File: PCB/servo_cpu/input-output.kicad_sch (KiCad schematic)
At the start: 1 part, among them J8 IO

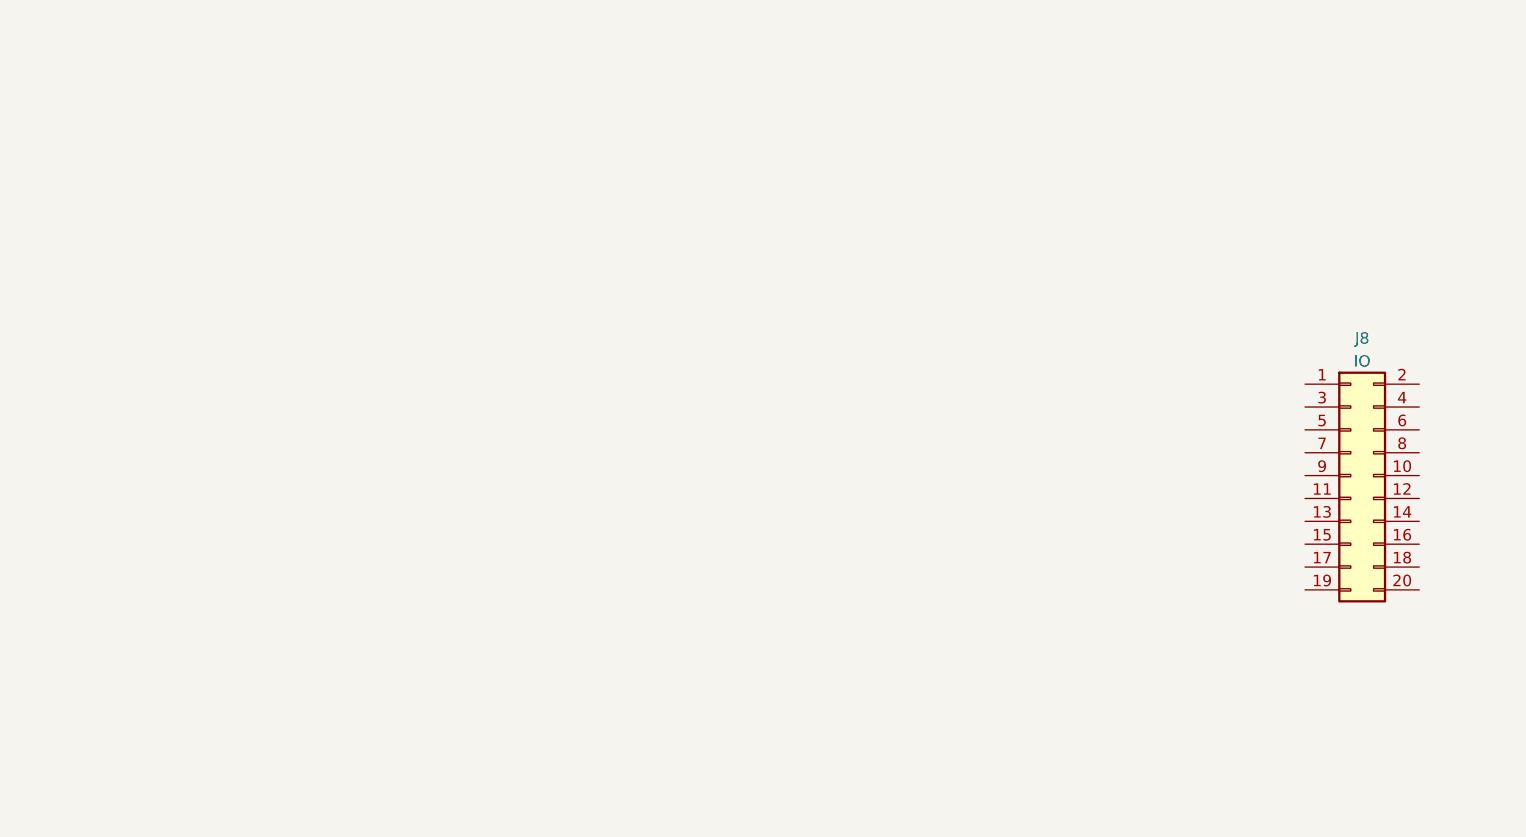
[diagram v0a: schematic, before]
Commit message: cpu pcb
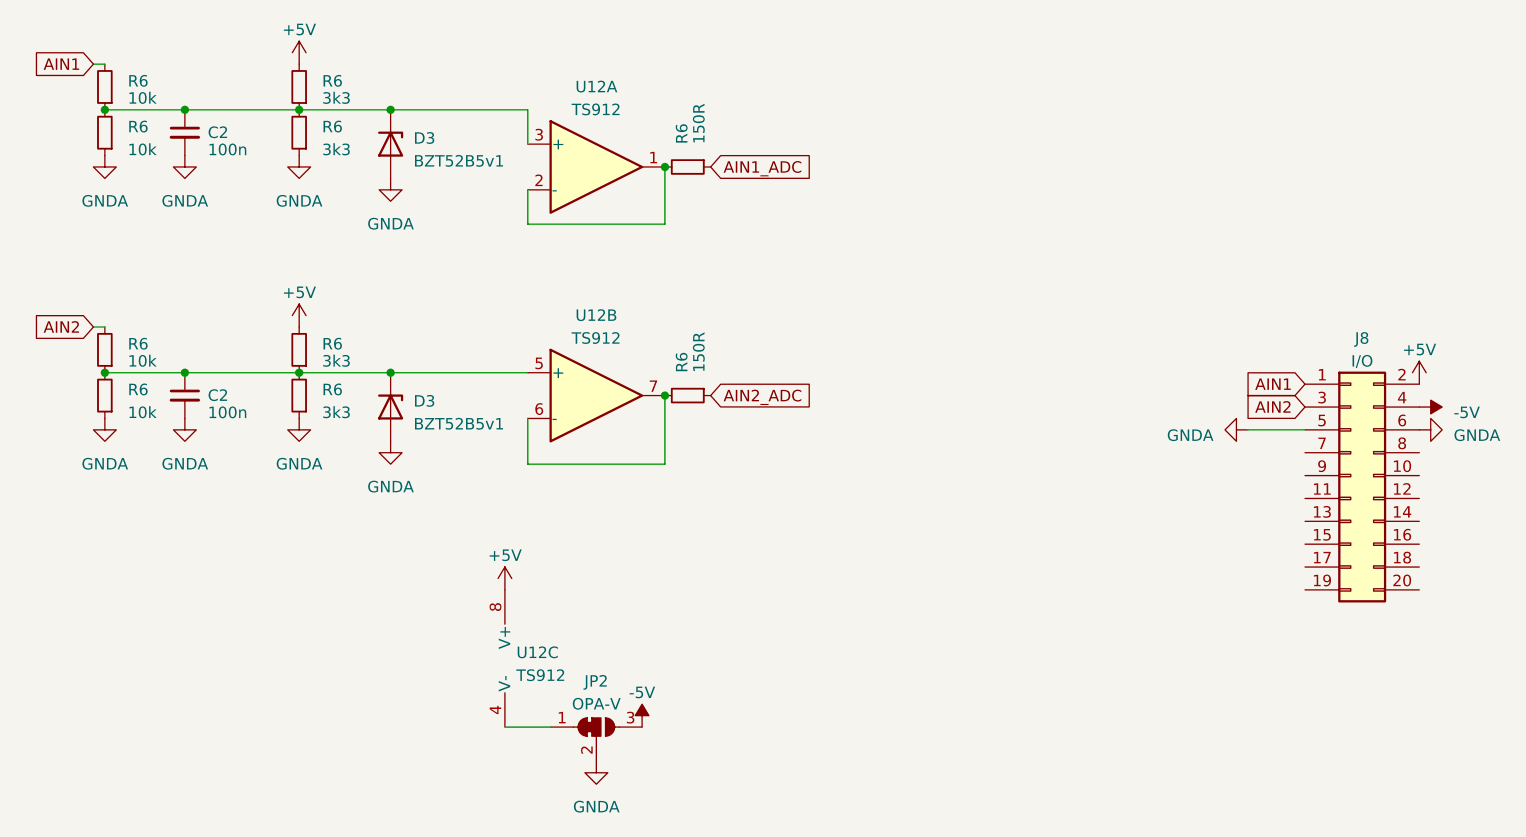
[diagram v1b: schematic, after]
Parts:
- added C2 (x2): 100n, symbol Device:C_Small
- added D3 (x2): BZT52B5v1, Diode_SMD:D_SOD-123F, symbol Diode:BZT52Bxx
- added JP2: OPA-V, Jumper:SolderJumper-3_P1.3mm_Bridged12_Pad1.0x1.5mm, symbol Jumper:SolderJumper_3_Bridged12
- added R6 (x2): 150R, symbol Device:R_Small
- added R6 (x4): 10k, symbol Device:R_Small
- added R6 (x4): 3k3, symbol Device:R_Small
- added U12: TS912, symbol Amplifier_Operational:TS912
- J8: value IO -> I/O
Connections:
- net AIN1: now reaches J8.1 (Pin_1)
- net AIN1: now also R6.2
- net +5V: now reaches J8.2 (Pin_2)
- net +5V: now also R6.2, R6.2, U12.8 (V+)
- net AIN2: now reaches J8.3 (Pin_3)
- net AIN2: now also R6.2
- net -5V: now reaches J8.4 (Pin_4)
- net -5V: now also JP2.3 (B)
- net GNDA: now reaches J8.5 (Pin_5)
- net GNDA: now also J8.6 (Pin_6), C2.2, C2.2, D3.2 (A), D3.2 (A), JP2.2 (C), R6.1, R6.1, R6.1, R6.1
- new net: C2.1, D3.1 (K), R6.1, R6.1, R6.2, R6.2, U12.3 (+)
- new net: R6.2, U12.6 (-), U12.7
- new net: JP2.1 (A), U12.4 (V-)
- new net: R6.2, U12.1, U12.2 (-)
- new net: C2.1, D3.1 (K), R6.1, R6.1, R6.2, R6.2, U12.5 (+)
- new net AIN1_ADC: R6.1
- new net AIN2_ADC: R6.1
